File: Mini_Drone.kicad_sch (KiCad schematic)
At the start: 38 parts, among them J1 Conn_01x02, Q1 AO3400A, Q2 AO3400A, Q3 AO3400A, Q4 AO3400A, U1 XIAO ESP32-S3, U2 MPU-6050

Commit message: good progress
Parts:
- U2: footprint Sensor_Motion:InvenSense_QFN-24_4x4mm_P0.5mm -> Drone_prj:InvenSense_QFN-24_4x4mm_P0.5mm
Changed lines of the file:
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@@
+		(length 2.54)
+		(shape round)
+		(at 195.58 116.84 180)
+		(fields_autoplaced yes)
+		(effects
+			(font
+				(size 1.27 1.27)
+			)
+			(justify right bottom)
+		)
+		(property "Netclass" "i2c_lines"
+			(at 196.2785 119.38 0)
+			(effects
+				(font
+					(size 1.27 1.27)
+				)
+				(justify left)
+			)
+		)
+		(property "Component Class" ""
+			(at -88.9 2.54 0)
+			(effects
+				(font
+					(size 1.27 1.27)
+					(italic yes)
+				)
+			)
+		)
+	)
+	(netclass_flag ""
 		(length 2.54)
 		(shape round)
@@
 		(property "Component Class" ""
 			(at -69.85 -11.43 0)
+			(effects
+				(font
+					(size 1.27 1.27)
+					(italic yes)
+				)
+			)
+		)
+	)
+	(netclass_flag ""
+		(length 2.54)
+		(shape round)
+		(at 193.04 114.3 0)
+		(fields_autoplaced yes)
+		(effects
+			(font
+				(size 1.27 1.27)
+			)
+			(justify left bottom)
+		)
+		(property "Netclass" "i2c_lines"
+			(at 193.7385 111.76 0)
+			(effects
+				(font
+					(size 1.27 1.27)
+				)
+				(justify left)
+			)
+		)
+		(property "Component Class" ""
+			(at -91.44 0 0)
 			(effects
 				(font
@@
 			)
 		)
-		(property "Footprint" "Sensor_Motion:InvenSense_QFN-24_4x4mm_P0.5mm"
+		(property "Footprint" "Drone_prj:InvenSense_QFN-24_4x4mm_P0.5mm"
 			(at 231.14 142.24 0)
 			(effects

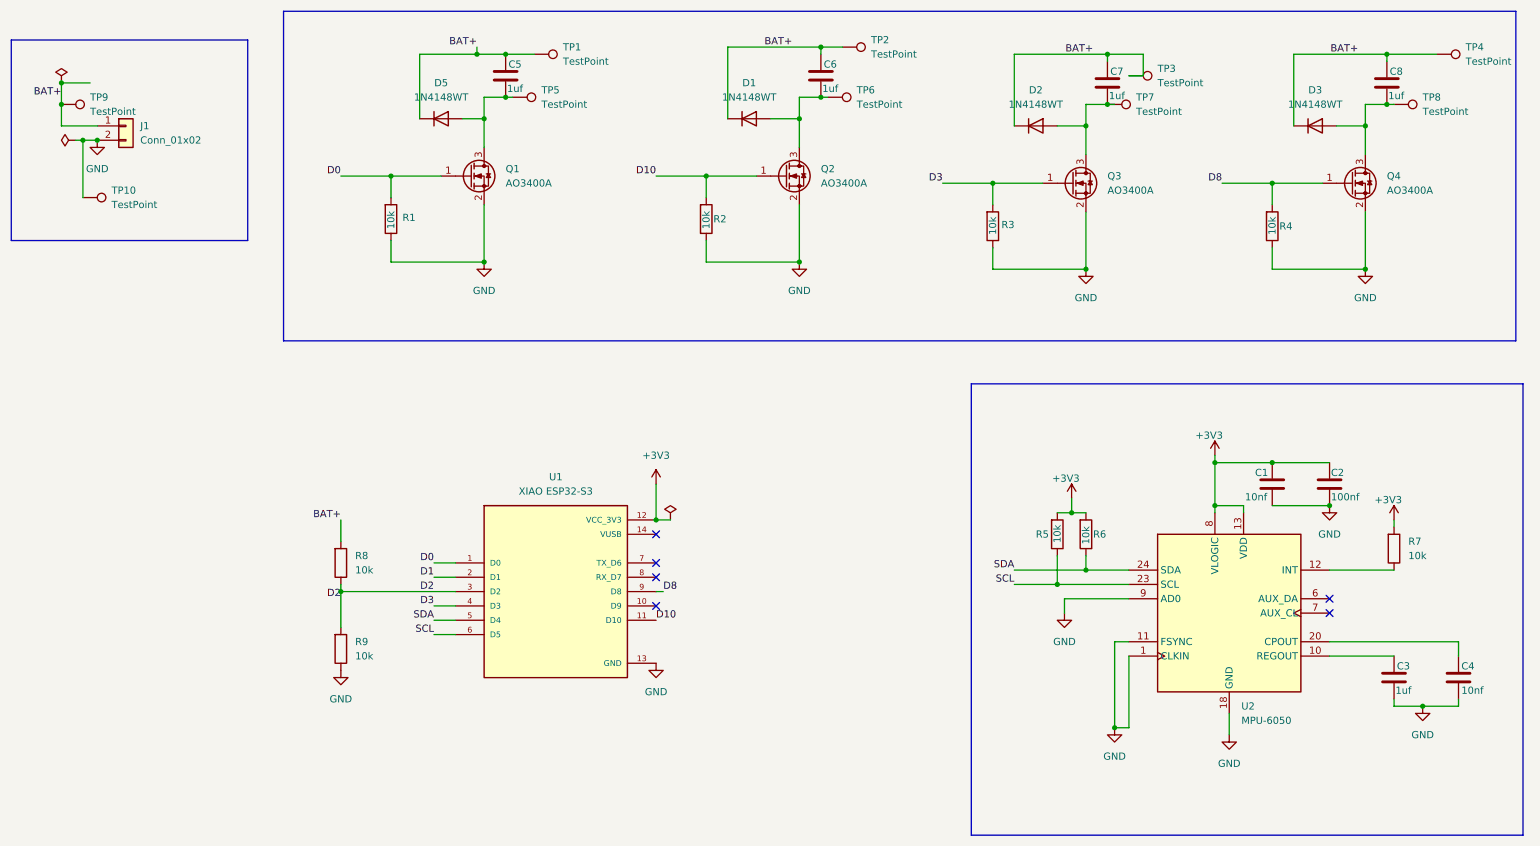
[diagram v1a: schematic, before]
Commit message: sch organized no error success
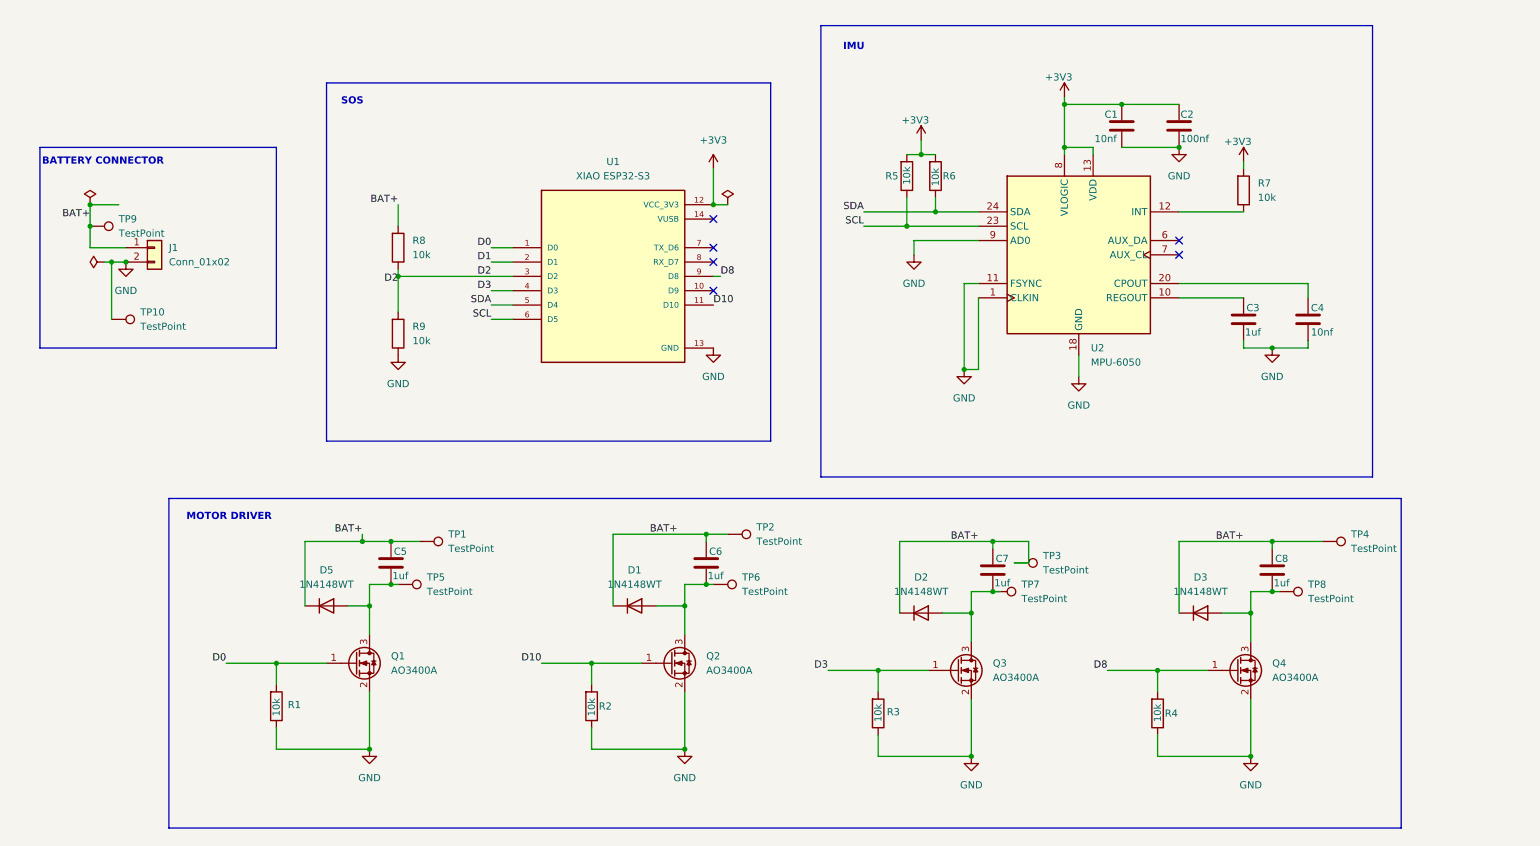
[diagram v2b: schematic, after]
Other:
- note added: "BATTERY CONNECTOR"
- note added: "IMU"
- note added: "MOTOR DRIVER"
- note added: "SOS"
- moved on the sheet: C1, C2, C3, C4, C5, C6, C7, C8, D1, D2, D3, D5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
